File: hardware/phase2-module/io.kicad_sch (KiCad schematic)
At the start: 6 parts, among them J1 XT60PW-M SLOT PWR, J4 XT60PW-M OUTPUT, J5 SLOT SIGNALS, J6 FAN, Q8 2N7002

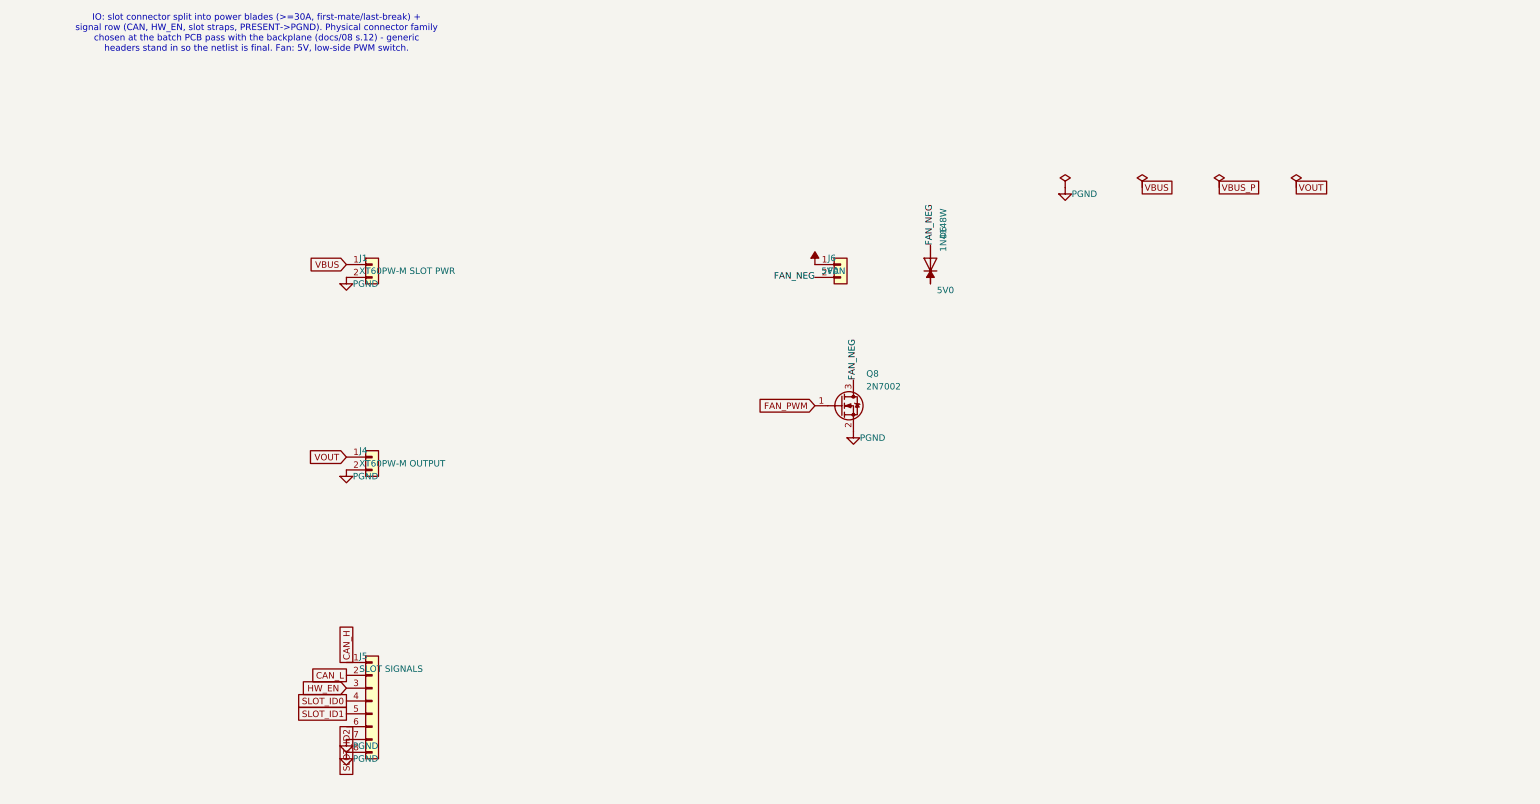
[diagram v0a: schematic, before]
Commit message: Add autosaved schematic files for power stage and auxiliary rails in phase2-module
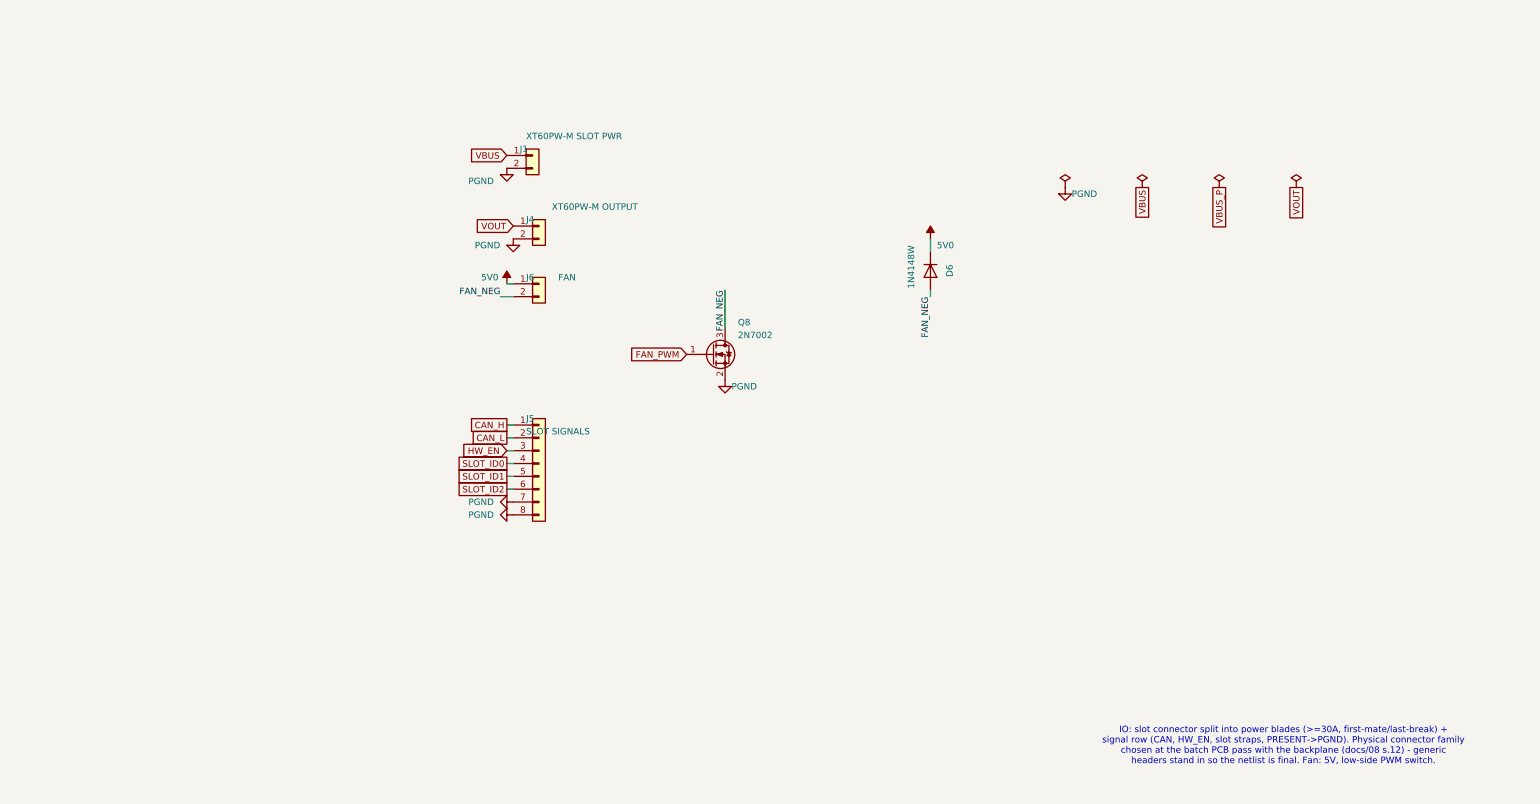
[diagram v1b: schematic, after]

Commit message: Refactor code structure for improved readability and maintainability
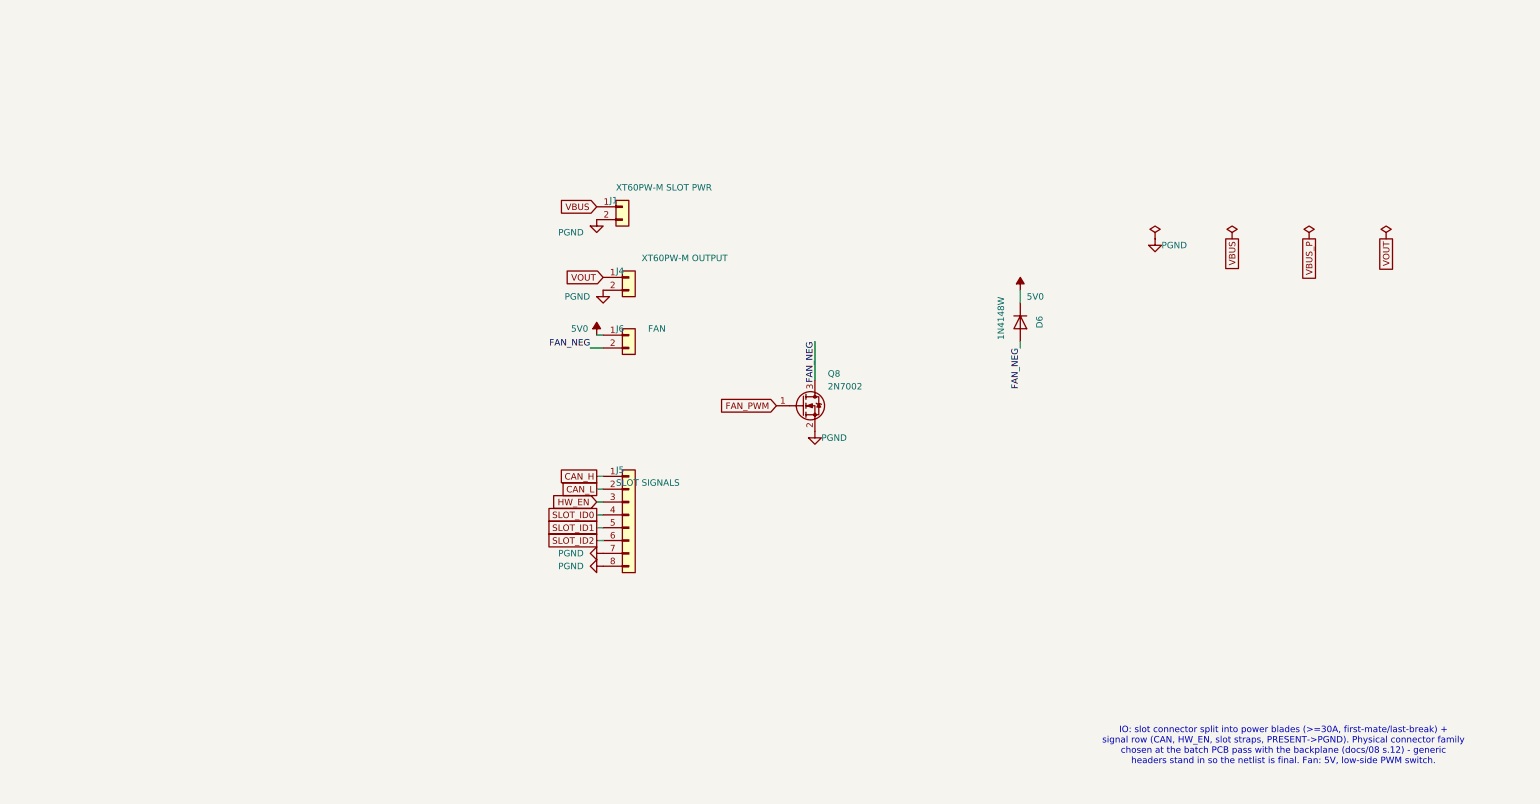
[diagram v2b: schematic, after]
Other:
- moved on the sheet: D6, J1, J4, J5, J6, Q8
